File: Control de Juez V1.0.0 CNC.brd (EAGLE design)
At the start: 35.5 x 67.3 mm, 21 parts, among them Q1 MMBT3904, U1 ATTINY412-SSNSOIC8_SA_SST_MCH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

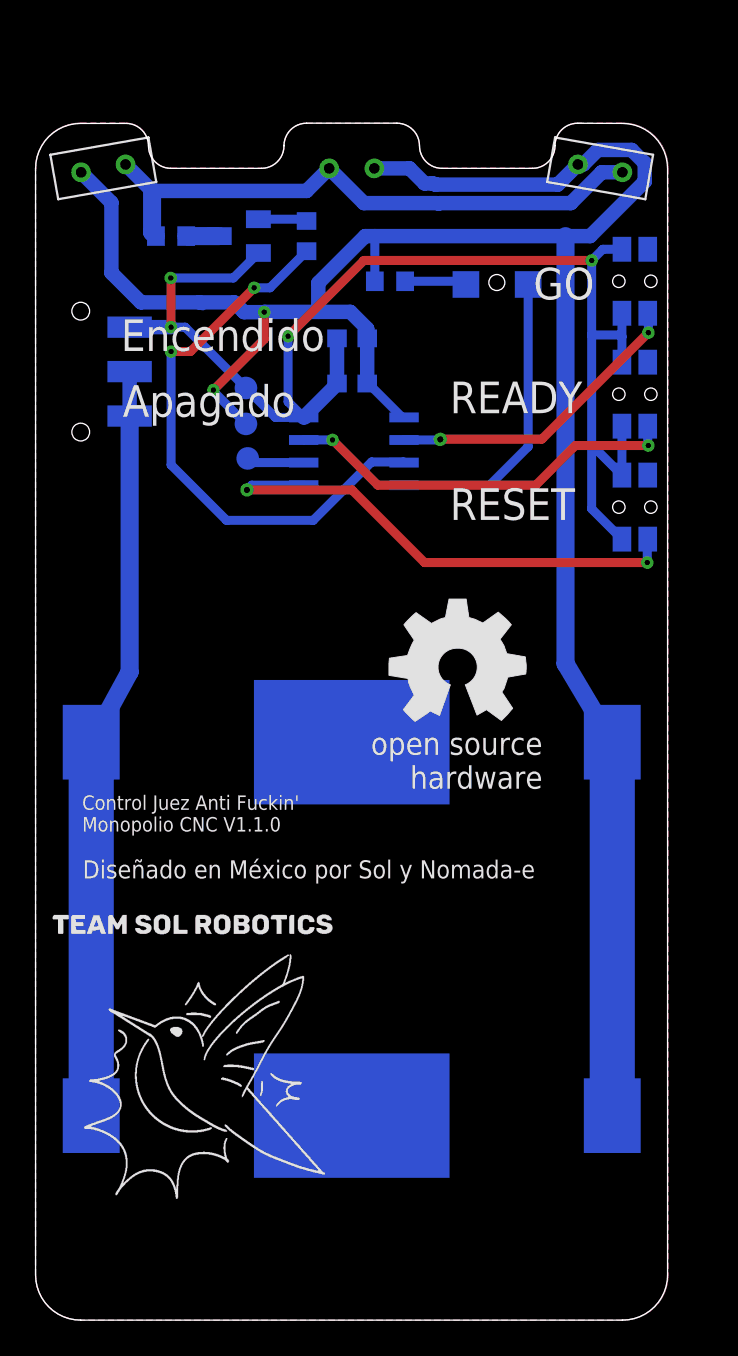
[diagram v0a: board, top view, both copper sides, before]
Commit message: Add files via upload
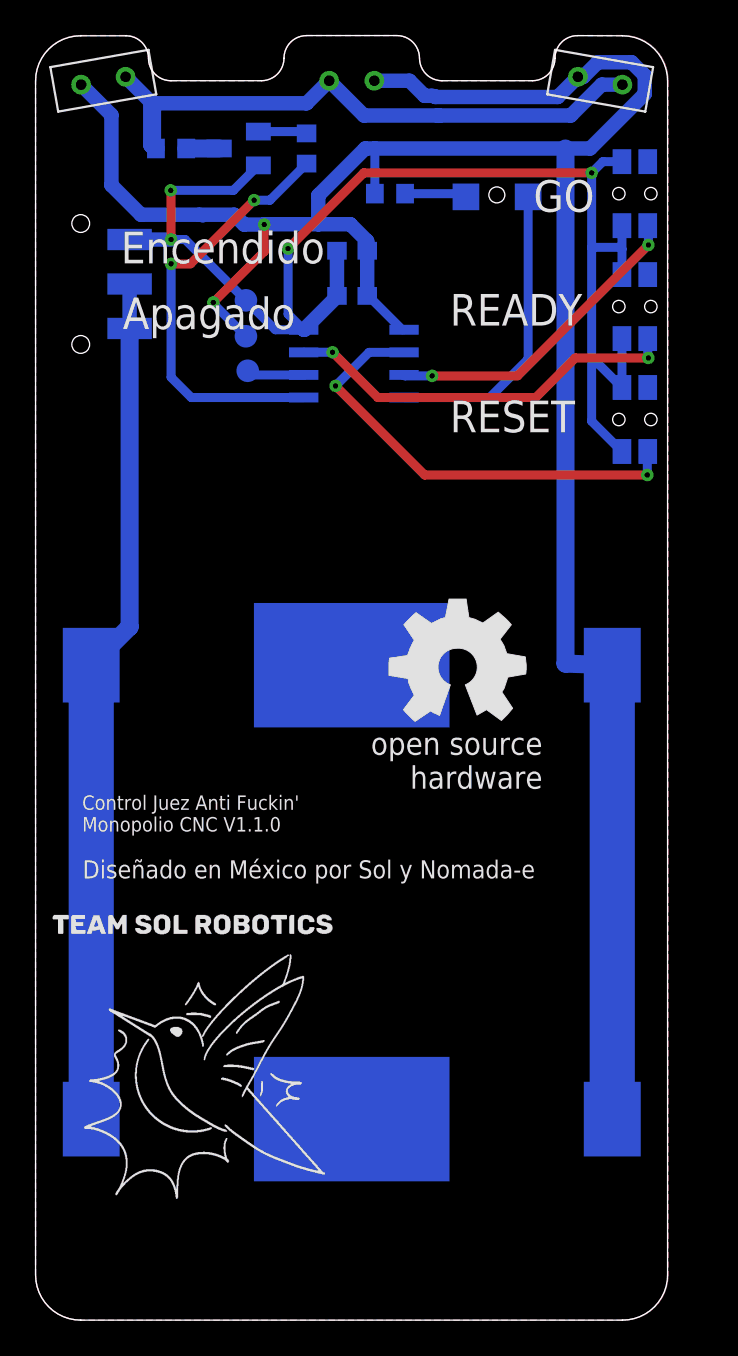
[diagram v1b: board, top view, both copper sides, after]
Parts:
- moved Q1 4.93 mm to (11.4, 65.9)
- moved R1 4.93 mm to (7.62, 65.9)
- moved R2 4.93 mm to (15.2, 65.9)
- moved C1 4.93 mm to (17.8, 57.6)
- moved C4 4.93 mm to (17.8, 60.1)
- moved GND 4.93 mm to (11.8, 57.3)
- moved GO 4.93 mm to (33.7, 63.3)
- moved LED1 4.93 mm to (31.8, 69.7)
- moved LED2 4.93 mm to (17.8, 69.7)
- moved LED3 4.93 mm to (3.81, 69.7)
- moved LED5 4.93 mm to (25.9, 63.2)
- moved R6 4.93 mm to (19.9, 63.3)
- moved READY 4.93 mm to (33.7, 50.6)
- moved RESET 4.93 mm to (33.7, 57.0)
- moved S1 4.93 mm to (2.54, 58.3)
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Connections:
- net LEDSMD renamed LEDSTATUS
- removed net LEDS: R2.2, U1.3
- removed net RST: RESET.2_1, RESET.2_2, U1.7
- new net LEDTRANSMISION: R2.2, U1.5
- new net RESET: READY.2_1, READY.2_2, U1.2
- net GO: now also U1.3; no longer U1.2
- net READY: now also RESET.2_1, RESET.2_2, U1.7; no longer READY.2_1, READY.2_2, U1.5
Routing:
- net LEDS: track 32.1 -> 0.00 mm, vias 2 -> 0
- net RESET: track 0.00 -> 25.6 mm, vias 0 -> 2
- net LEDTRANSMISION: track 0.00 -> 24.3 mm, vias 0 -> 2
- net RST: track 22.5 -> 0.00 mm, vias 2 -> 0
- net +5V: track 129.4 -> 136.3 mm
- net READY: track 28.8 -> 22.5 mm
- net N$2: track 42.9 -> 47.9 mm
- net LEDSTATUS: track 12.2 -> 17.0 mm
- net GO: track 17.3 -> 17.9 mm
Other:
- board size 35.5 x 67.3 mm -> 35.5 x 72.2 mm

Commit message: Add files via upload
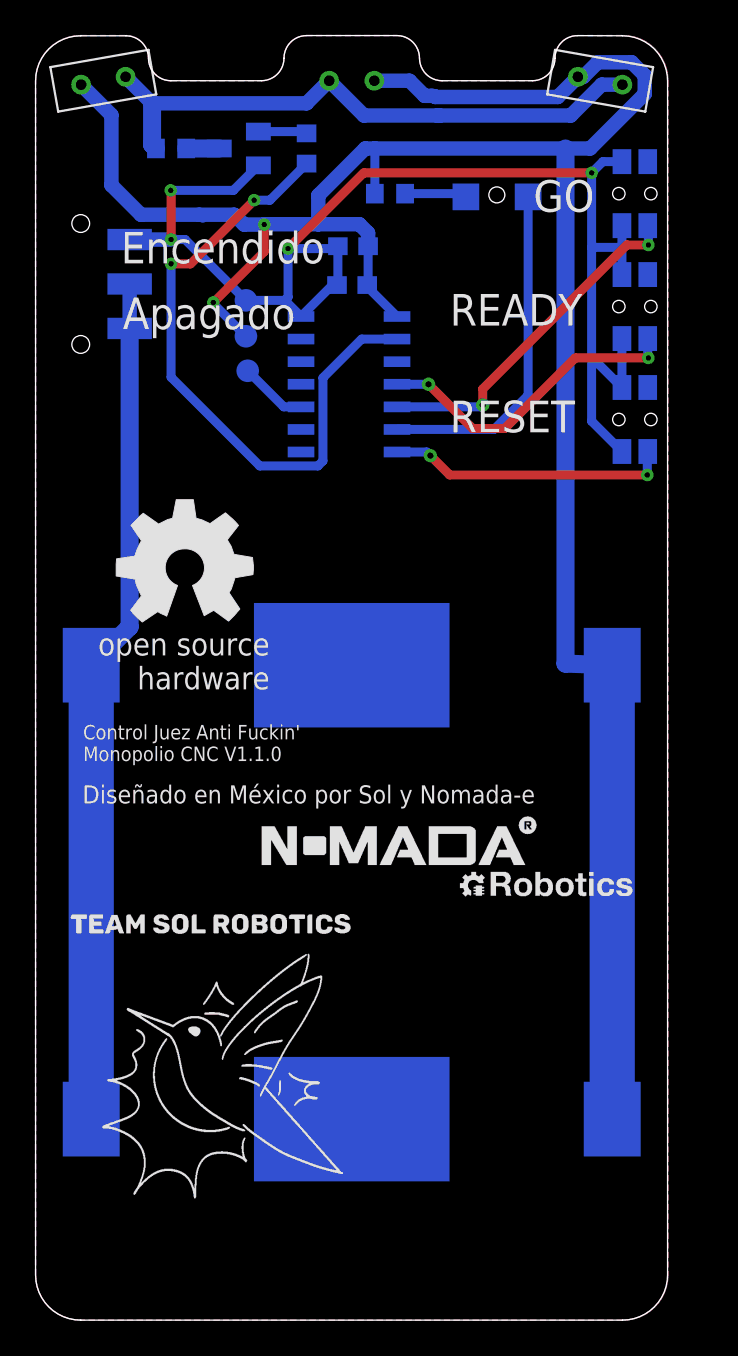
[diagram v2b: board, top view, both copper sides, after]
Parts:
- removed U1: ATTINY412-SSNSOIC8_SA_SST_MCH-M, attiny412:SOIC8_SA_SST_MCH-M
- added U2: ATTINY1614-SSNR, Attiny1614:SOIC14_SL_MCH
- moved GOLD_ORB_SM1 16.3 mm to (8.37, 42.3)
- moved C1 0.61 mm to (17.8, 58.2)
- moved C4 0.26 mm to (17.9, 60.4)
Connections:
- removed net N$1: U1.6, UPDI.TP
- new net UPDI: U2.10, UPDI.TP
- net +5V: now also U2.1; no longer U1.1
- net GND: now also U2.14; no longer U1.8
- net GO: now also U2.5; no longer U1.3
- net LEDSTATUS: now also U2.6; no longer U1.4
- net LEDTRANSMISION: now also U2.2; no longer U1.5
- net READY: now also U2.4; no longer U1.7
- net RESET: now also U2.7; no longer U1.2
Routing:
- net LEDTRANSMISION: track 24.3 -> 36.8 mm
- net RESET: track 25.6 -> 15.9 mm
- net READY: track 22.5 -> 17.9 mm
- net UPDI: track 0.00 -> 3.84 mm
- net N$1: track 3.25 -> 0.00 mm
- net LEDSTATUS: track 17.0 -> 19.3 mm
- net GO: track 17.9 -> 19.5 mm
- net +5V: track 136.3 -> 135.7 mm
